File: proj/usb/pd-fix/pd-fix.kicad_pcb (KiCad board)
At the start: 2 copper layers, 10 x 10 mm, 9 parts, among them J1 USB_C_Receptacle_PowerOnly_6P, J2 Conn_01x02_Pin, U1 CH221K

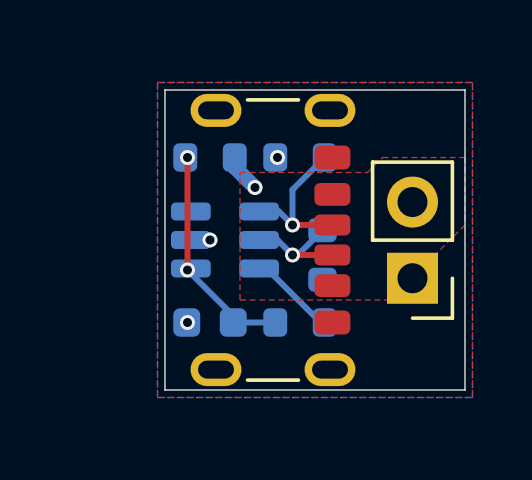
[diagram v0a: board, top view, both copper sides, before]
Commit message: -
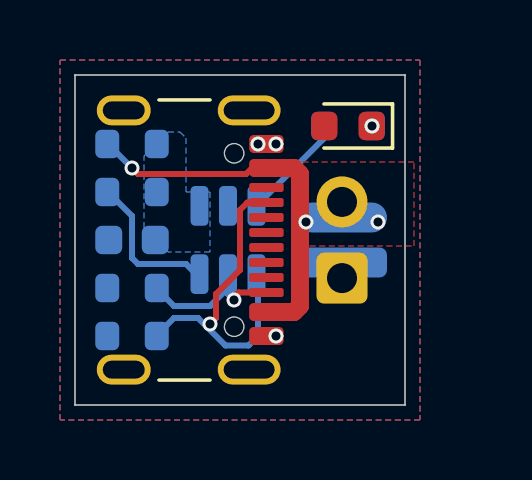
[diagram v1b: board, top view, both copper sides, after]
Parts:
- removed G***: LOGO, LOGO
- added D1: PG, LED_SMD:LED_0603_1608Metric, F.Cu at (103.6, 96.2)
- added R5: 10k, Resistor_SMD:R_0603_1608Metric, B.Cu at (103.6, 96.2)
- J1: value USB_C_Receptacle_PowerOnly_6P -> USB_C_Receptacle_USB2.0_16P; footprint Connector_USB:USB_C_Receptacle_GCT_USB4125-xx-x_6P_TopMnt_Horizontal -> Connector_USB:USB_C_Receptacle_GCT_USB4105-xx-A_16P_TopMnt_Horizontal
- J2: footprint Connector_PinHeader_2.54mm:PinHeader_1x02_P2.54mm_Vertical -> Library:SolderPad_2P; moved to B.Cu
- moved R2 8.17 mm to (96.4, 103.2)
- moved R4 7.09 mm to (96.4, 98.4), turned to 180 degrees
- moved R3 6.44 mm to (96.4, 101.6), turned to 180 degrees
- moved C1 3.78 mm to (96.4, 100.0)
- moved J1 2.80 mm to (97.2, 100.0)
- moved J2 2.67 mm to (103.4, 100.0), turned to 0 degrees
- moved R1 2.64 mm to (96.4, 96.8), turned to 0 degrees
- moved U1 0.10 mm to (99.6, 100.0), turned to -90 degrees
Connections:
- U1 pad 3: unconnected-(U1-PG#-Pad3) -> Net-(U1-PG#)
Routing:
- net VBUS: track 1.28 -> 12.6 mm, vias 1 -> 3
- net VDD: track 7.53 -> 0.00 mm, vias 2 -> 0
- net CC1: track 5.07 -> 11.4 mm
- net Net-(U1-PG#): track 0.00 -> 3.78 mm
- net Net-(U1-CFG): track 2.68 -> 5.03 mm
- net CC2: track 3.74 -> 5.07 mm
- net Net-(D1-K): vias 0 -> 1
- added copper zone on B.Cu, net VDD
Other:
- board size 10 x 10 mm -> 11 x 11 mm
- board text added: "103 5 473 12 203 9 104 15 204 20"
- board text added: "1k ~0.28W CFG 1u 4k7 4k7"
- board text added: "@Mcbe Eringi"
- board text added: "PD TRG FIXED"
- board text removed: "PD FIX"
